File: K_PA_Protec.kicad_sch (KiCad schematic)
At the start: 89 parts, among them IC1 MCP23017_SO, J1 IDC 10 Straight, J10 MH2, J11 MH3, J12 MH4, J13 MH5, J14 MH6, J2 Molex KK 4, J3 IDC 10 Straight, J4 Molex KK 2, J5 IDC 10 Straight, J6 Molex KK 2, J7 Molex KK 3, J8 Molex KK 4, J9 MH1, Q1 2N7002, Q2 2N7002, SW1 RotaryEncoder_Dual_Switch, U1 LM339, U2 74HC02, U3 74HC21, U4 LM1117-3.3, U6 YAAJ_DCDC_StepDown_LM2596

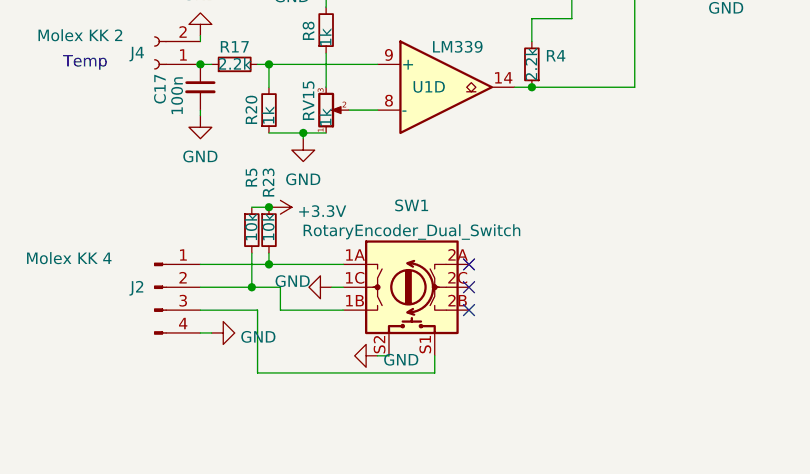
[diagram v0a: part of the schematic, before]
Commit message: routing, first stage
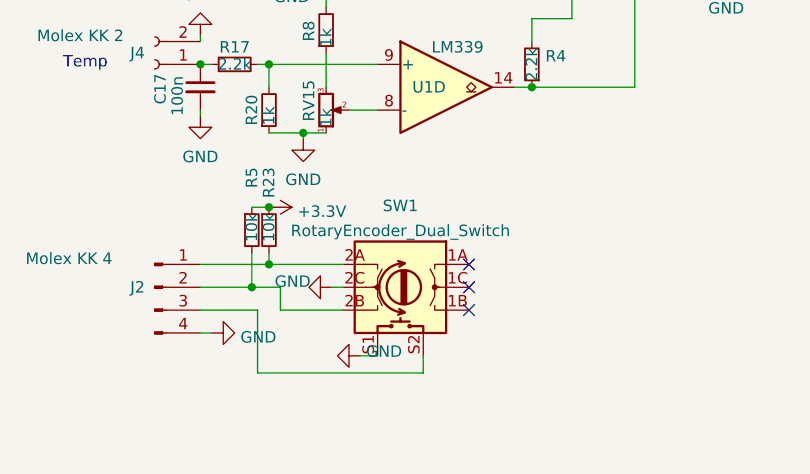
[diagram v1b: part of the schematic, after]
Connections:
- net GND: now also SW1.2C, SW1.S1; no longer SW1.1C, SW1.S2
- net at J2.1 (Pin_1), R23.2: now also SW1.2A; no longer SW1.1A
- net at J2.2 (Pin_2), R5.2: now also SW1.2B; no longer SW1.1B
- net at J2.3 (Pin_3): now also SW1.S2; no longer SW1.S1
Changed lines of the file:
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@@
     (stroke (width 0) (type default) (color 0 0 0 0))
   )
-  (wire (pts (xy 55.245 186.69) (xy 56.515 186.69))
+  (wire (pts (xy 55.245 186.69) (xy 53.34 186.69))
     (stroke (width 0) (type default) (color 0 0 0 0))
   )
@@
     (stroke (width 0) (type default) (color 0 0 0 0))
   )
-  (wire (pts (xy 61.595 188.595) (xy 61.595 186.69))
-    (stroke (width 0) (type default) (color 0 0 0 0))
-  )
   (wire (pts (xy 131.445 17.78) (xy 132.715 17.78))
     (stroke (width 0) (type default) (color 0 0 0 0))
   )
+  (wire (pts (xy 41.91 188.595) (xy 60.325 188.595))
+    (stroke (width 0) (type default) (color 0 0 0 0))
+  )
   (wire (pts (xy 133.35 86.995) (xy 133.35 87.63))
     (stroke (width 0) (type default) (color 0 0 0 0))
@@
     (stroke (width 0) (type default) (color 0 0 0 0))
   )
+  (wire (pts (xy 60.325 186.69) (xy 60.325 188.595))
+    (stroke (width 0) (type default) (color 0 0 0 0))
+  )
   (wire (pts (xy 34.925 33.02) (xy 34.925 34.29))
     (stroke (width 0) (type default) (color 0 0 0 0))
@@
   )
   (wire (pts (xy 165.1 150.495) (xy 170.18 150.495))
-    (stroke (width 0) (type default) (color 0 0 0 0))
-  )
-  (wire (pts (xy 41.91 188.595) (xy 61.595 188.595))
     (stroke (width 0) (type default) (color 0 0 0 0))
   )
@@
     (pin "1")
   )
-  (symbol (lib_id "RotaryEncoder_Dual_Alps_EC11E-Switch_Vertical_H20mm:RotaryEncoder_Dual_Switch") (at 59.055 179.07 0) (unit 1)
-    (in_bom yes) (on_board yes) (fields_autoplaced)
-    (property "Reference" "SW1" (id 0) (at 59.055 170.0235 0))
-    (property "Value" "RotaryEncoder_Dual_Switch" (id 1) (at 59.055 172.7986 0))
-    (property "Footprint" "RotaryEncoder_Dual_Alps_EC11E-Switch_Vertical_H20mm:RotaryEncoder_Dual_Alps_EC11E-Switch_Vertical_H20mm" (id 2) (at 55.245 175.006 0)
-      (effects (font (size 1.27 1.27)) hide)
-    )
-    (property "Datasheet" "~" (id 3) (at 59.055 172.466 0)
+  (symbol (lib_id "RotaryEncoder_Dual_Alps_EC11E-Switch_Vertical_H20mm:RotaryEncoder_Dual_Switch") (at 57.785 179.07 0) (mirror y) (unit 1)
+    (in_bom yes) (on_board yes) (fields_autoplaced)
+    (property "Reference" "SW1" (id 0) (at 57.785 170.0235 0))
+    (property "Value" "RotaryEncoder_Dual_Switch" (id 1) (at 57.785 172.7986 0))
+    (property "Footprint" "RotaryEncoder_Dual_Alps_EC11E-Switch_Vertical_H20mm:RotaryEncoder_Dual_Alps_EC11E-Switch_Vertical_H20mm" (id 2) (at 61.595 175.006 0)
+      (effects (font (size 1.27 1.27)) hide)
+    )
+    (property "Datasheet" "~" (id 3) (at 57.785 172.466 0)
       (effects (font (size 1.27 1.27)) hide)
     )
@@
     (pin "9")
   )
-  (symbol (lib_id "power:GND") (at 55.245 186.69 270) (unit 1)
-    (in_bom yes) (on_board yes) (fields_autoplaced)
-    (property "Reference" "#PWR0173" (id 0) (at 48.895 186.69 0)
-      (effects (font (size 1.27 1.27)) hide)
-    )
-    (property "Value" "GND" (id 1) (at 55.88 187.169 90)
+  (symbol (lib_id "power:GND") (at 53.34 186.69 270) (mirror x) (unit 1)
+    (in_bom yes) (on_board yes) (fields_autoplaced)
+    (property "Reference" "#PWR0173" (id 0) (at 46.99 186.69 0)
+      (effects (font (size 1.27 1.27)) hide)
+    )
+    (property "Value" "GND" (id 1) (at 53.975 186.211 90)
       (effects (font (size 1.27 1.27)) (justify left))
     )
-    (property "Footprint" "" (id 2) (at 55.245 186.69 0)
-      (effects (font (size 1.27 1.27)) hide)
-    )
-    (property "Datasheet" "" (id 3) (at 55.245 186.69 0)
-      (effects (font (size 1.27 1.27)) hide)
-    )
+    (property "Footprint" "" (id 2) (at 53.34 186.69 0)
+      (effects (font (size 1.27 1.27)) hide)
+    )
+    (property "Datasheet" "" (id 3) (at 53.34 186.69 0)
+      (effects (font (size 1.27 1.27)) hide)
+    )
